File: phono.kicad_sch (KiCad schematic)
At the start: 63 parts, among them J1 Power +30V, J2 R Phono in, J3 L Phono in, J4 R Phono out, J5 L Phono out, Q1 2N2222, Q2 2N2222, Q3 2N2222, Q4 2N2222, Q5 2N2222, Q6 2N2222

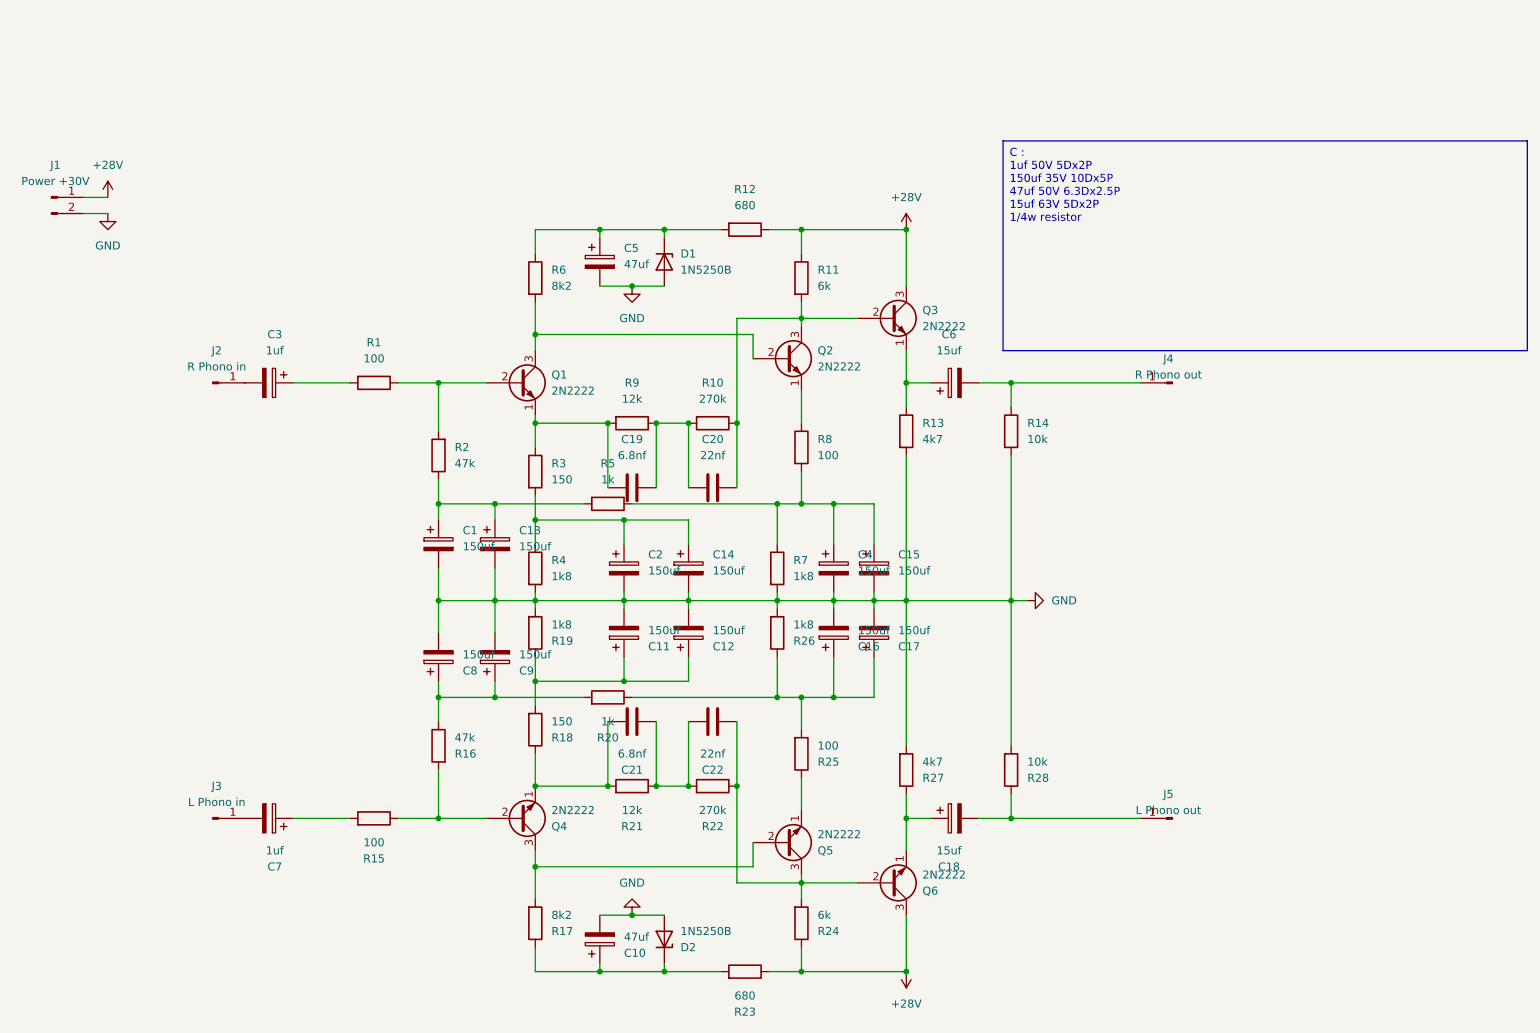
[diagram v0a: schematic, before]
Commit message: Add files via upload
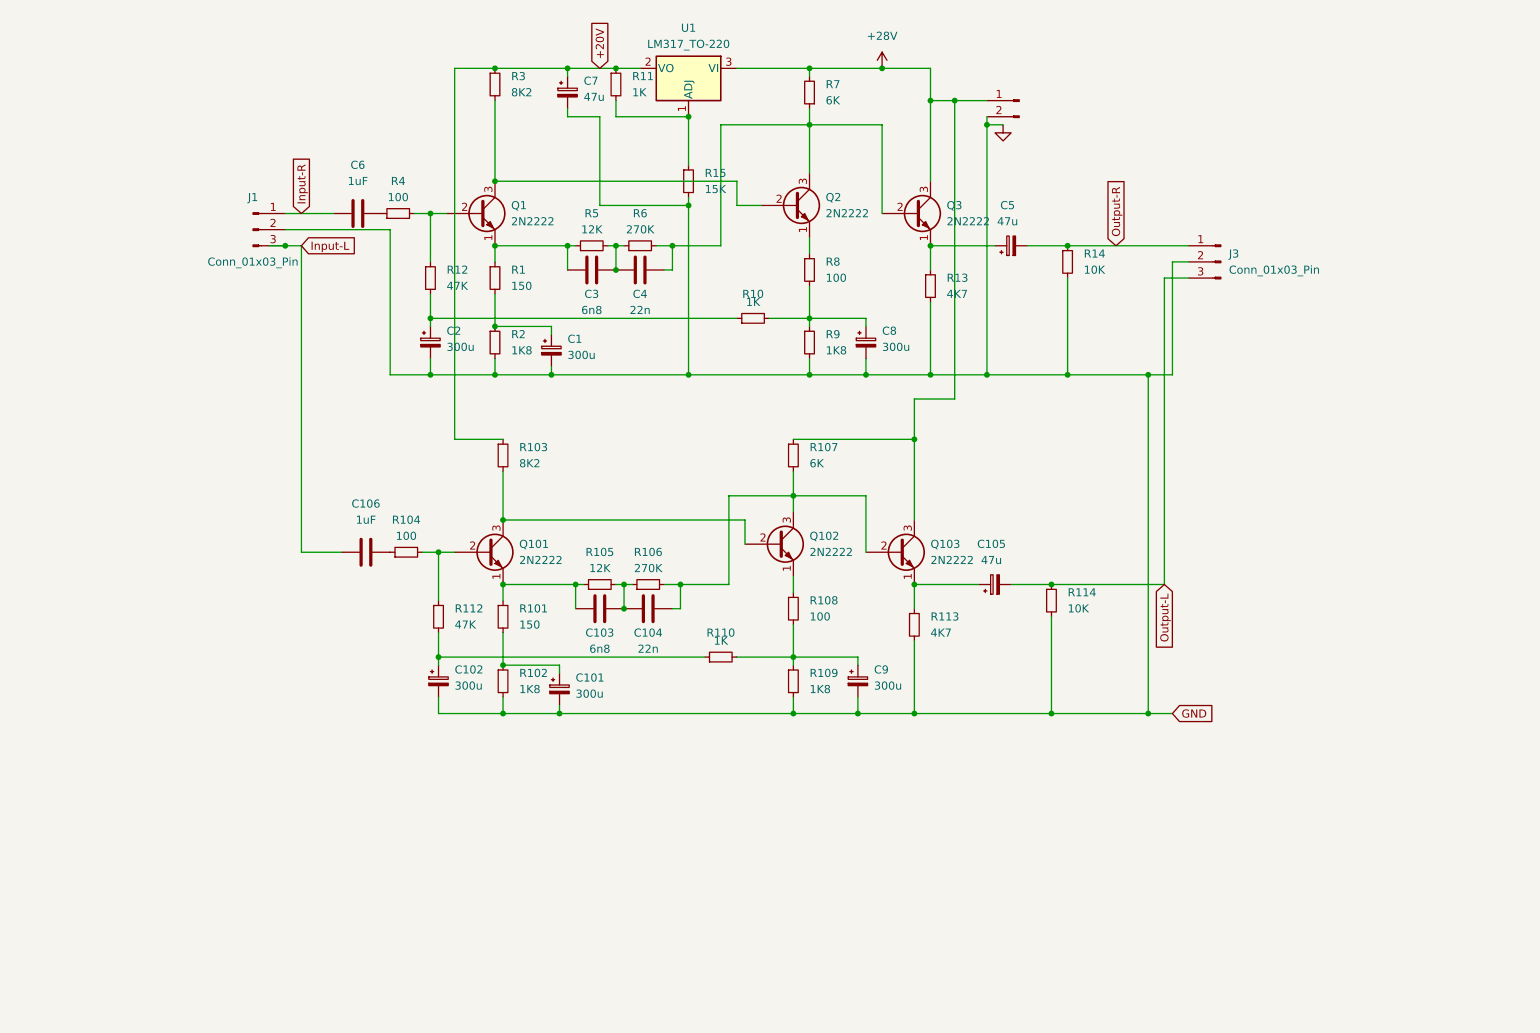
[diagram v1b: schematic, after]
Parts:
- removed C1, C11, C12, C13, C14, C15, C16, C17, C2, C4, C8, C9: 150uf, Capacitor_THT:CP_Radial_D10.0mm_P5.00mm, symbol Device:C_Polarized
- removed C10, C5: 47uf, Capacitor_THT:CP_Radial_D6.3mm_P2.50mm, symbol Device:C_Polarized
- removed C18, C6: 15uf, Capacitor_THT:CP_Radial_D5.0mm_P2.00mm, symbol Device:C_Polarized
- removed C19, C21: 6.8nf, Capacitor_THT:C_Rect_L7.0mm_W2.0mm_P5.00mm, symbol Device:C
- removed C20, C22: 22nf, Capacitor_THT:C_Rect_L7.0mm_W2.0mm_P5.00mm, symbol Device:C
- removed C3, C7: 1uf, Capacitor_THT:CP_Radial_D4.0mm_P2.00mm, symbol Device:C_Polarized
- removed D1, D2: 1N5250B, Diode_THT:D_DO-41_SOD81_P10.16mm_Horizontal, symbol Diode:1N47xxA
- removed J1: Power +30V, Connector_Wire:SolderWire-2sqmm_1x02_P7.8mm_D2mm_OD3.9mm, symbol Connector:Conn_01x02_Pin
- removed J2: R Phono in, Connector_Wire:SolderWire-2sqmm_1x01_D2mm_OD3.9mm, symbol Connector:Conn_01x01_Pin
- removed J3: L Phono in, Connector_Wire:SolderWire-2sqmm_1x01_D2mm_OD3.9mm, symbol Connector:Conn_01x01_Pin
- removed J4: R Phono out, Connector_Wire:SolderWire-2sqmm_1x01_D2mm_OD3.9mm, symbol Connector:Conn_01x01_Pin
- removed J5: L Phono out, Connector_Wire:SolderWire-2sqmm_1x01_D2mm_OD3.9mm, symbol Connector:Conn_01x01_Pin
- removed Q1, Q2, Q3, Q4, Q5, Q6: 2N2222, Package_TO_SOT_THT:TO-18-3, symbol Transistor_BJT:BC107
- removed R1, R15, R25, R8: 100, Resistor_THT:R_Axial_DIN0207_L6.3mm_D2.5mm_P10.16mm_Horizontal, symbol Device:R
- removed R10, R22: 270k, Resistor_THT:R_Axial_DIN0207_L6.3mm_D2.5mm_P10.16mm_Horizontal, symbol Device:R
- removed R11, R24: 6k, Resistor_THT:R_Axial_DIN0207_L6.3mm_D2.5mm_P10.16mm_Horizontal, symbol Device:R
- removed R12, R23: 680, Resistor_THT:R_Axial_DIN0207_L6.3mm_D2.5mm_P10.16mm_Horizontal, symbol Device:R
- removed R13, R27: 4k7, Resistor_THT:R_Axial_DIN0207_L6.3mm_D2.5mm_P10.16mm_Horizontal, symbol Device:R
- removed R14, R28: 10k, Resistor_THT:R_Axial_DIN0207_L6.3mm_D2.5mm_P10.16mm_Horizontal, symbol Device:R
- removed R16, R2: 47k, Resistor_THT:R_Axial_DIN0207_L6.3mm_D2.5mm_P10.16mm_Horizontal, symbol Device:R
- removed R17, R6: 8k2, Resistor_THT:R_Axial_DIN0207_L6.3mm_D2.5mm_P10.16mm_Horizontal, symbol Device:R
- removed R18, R3: 150, Resistor_THT:R_Axial_DIN0207_L6.3mm_D2.5mm_P10.16mm_Horizontal, symbol Device:R
- removed R19, R26, R4, R7: 1k8, Resistor_THT:R_Axial_DIN0207_L6.3mm_D2.5mm_P10.16mm_Horizontal, symbol Device:R
- removed R20, R5: 1k, Resistor_THT:R_Axial_DIN0207_L6.3mm_D2.5mm_P10.16mm_Horizontal, symbol Device:R
- removed R21, R9: 12k, Resistor_THT:R_Axial_DIN0207_L6.3mm_D2.5mm_P10.16mm_Horizontal, symbol Device:R
- added C1, C101, C102, C2, C8, C9: 300u, Capacitor_THT:CP_Radial_D10.0mm_P5.00mm, symbol Device:C_Polarized_Small
- added C103, C3: 6n8, Capacitor_THT:C_Axial_L3.8mm_D2.6mm_P10.00mm_Horizontal, symbol Device:C
- added C104, C4: 22n, Capacitor_THT:C_Axial_L3.8mm_D2.6mm_P10.00mm_Horizontal, symbol Device:C
- added C105, C5, C7: 47u, Capacitor_THT:CP_Radial_D10.0mm_P5.00mm, symbol Device:C_Polarized_Small
- added C106, C6: 1uF, Capacitor_THT:C_Axial_L3.8mm_D2.6mm_P10.00mm_Horizontal, symbol Device:C
- added J1, J3: Conn_01x03_Pin, TerminalBlock:TerminalBlock_bornier-3_P5.08mm, symbol Connector:Conn_01x03_Pin
- added J2: Conn_01x02_Pin, TerminalBlock:TerminalBlock_bornier-2_P5.08mm, symbol Connector:Conn_01x02_Pin
- added Q1, Q101, Q102, Q103, Q2, Q3: 2N2222, Package_TO_SOT_THT:TO-39-3, symbol Transistor_BJT:2N2219
- added R1, R101: 150, Resistor_THT:R_Axial_DIN0207_L6.3mm_D2.5mm_P10.16mm_Horizontal, symbol Device:R_Small
- added R10, R11, R110: 1K, Resistor_THT:R_Axial_DIN0207_L6.3mm_D2.5mm_P10.16mm_Horizontal, symbol Device:R_Small
- added R102, R109, R2, R9: 1K8, Resistor_THT:R_Axial_DIN0207_L6.3mm_D2.5mm_P10.16mm_Horizontal, symbol Device:R_Small
- added R103, R3: 8K2, Resistor_THT:R_Axial_DIN0207_L6.3mm_D2.5mm_P10.16mm_Horizontal, symbol Device:R_Small
- added R104, R108, R4, R8: 100, Resistor_THT:R_Axial_DIN0207_L6.3mm_D2.5mm_P10.16mm_Horizontal, symbol Device:R_Small
- added R105, R5: 12K, Resistor_THT:R_Axial_DIN0207_L6.3mm_D2.5mm_P10.16mm_Horizontal, symbol Device:R_Small
- added R106, R6: 270K, Resistor_THT:R_Axial_DIN0207_L6.3mm_D2.5mm_P10.16mm_Horizontal, symbol Device:R_Small
- added R107, R7: 6K, Resistor_THT:R_Axial_DIN0207_L6.3mm_D2.5mm_P10.16mm_Horizontal, symbol Device:R_Small
- added R112, R12: 47K, Resistor_THT:R_Axial_DIN0207_L6.3mm_D2.5mm_P10.16mm_Horizontal, symbol Device:R_Small
- added R113, R13: 4K7, Resistor_THT:R_Axial_DIN0207_L6.3mm_D2.5mm_P10.16mm_Horizontal, symbol Device:R_Small
- added R114, R14: 10K, Resistor_THT:R_Axial_DIN0207_L6.3mm_D2.5mm_P10.16mm_Horizontal, symbol Device:R_Small
- added R15: 15K, Resistor_THT:R_Axial_DIN0207_L6.3mm_D2.5mm_P10.16mm_Horizontal, symbol Device:R_Small
- added U1: LM317_TO-220, Package_TO_SOT_THT:TO-220-3_Vertical, symbol Regulator_Linear:LM317_TO-220
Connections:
- net +28V: now also J2.1 (Pin_1), Q103.3 (C), Q3.3 (C), R107.1, R7.2, U1.3 (VI)
- net GND: now also C1.2, C101.2, C102.2, C2.2, C7.2, C8.2, C9.2, J1.2 (Pin_2), J2.2 (Pin_2), J3.2 (Pin_2), R102.2, R109.2, R113.2, R114.2, R13.2, R14.2, R15.2, R2.2, R9.2
- new net: C106.2, R104.1
- new net: Q101.2 (B), R104.2, R112.1
- new net: C1.1, R1.2, R2.1
- new net: Q2.1 (E), R8.1
- new net: Q1.3 (C), Q2.2 (B), R3.2
- new net: C4.2, Q2.3 (C), Q3.2 (B), R6.2, R7.1
- new net: R11.2, R15.1, U1.1 (ADJ)
- new net: C2.1, R10.1, R12.2
- new net: C8.1, R10.2, R8.2, R9.1
- new net: C3.1, Q1.1 (E), R1.1, R5.1
- new net: C3.2, C4.1, R5.2, R6.1
- new net: C103.2, C104.1, R105.2, R106.1
- new net: C104.2, Q102.3 (C), Q103.2 (B), R106.2, R107.2
- new net: C105.1, Q103.1 (E), R113.1
- new net: C5.1, Q3.1 (E), R13.1
- new net: C6.2, R4.1
- new net: C103.1, Q101.1 (E), R101.1, R105.1
- new net: Q101.3 (C), Q102.2 (B), R103.2
- new net: C101.1, R101.2, R102.1
- new net: Q1.2 (B), R12.1, R4.2
- new net: C102.1, R110.1, R112.2
- new net: C9.1, R108.2, R109.1, R110.2
- new net: Q102.1 (E), R108.1
- new net +20V: C7.1, R103.1, R11.1, R3.1, U1.2 (VO)
- new net Input-L: C106.1, J1.3 (Pin_3)
- new net Input-R: C6.1, J1.1 (Pin_1)
- new net Output-L: C105.2, J3.3 (Pin_3), R114.1
- new net Output-R: C5.2, J3.1 (Pin_1), R14.1
